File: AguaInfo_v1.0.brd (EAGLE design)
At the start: 100 x 80 mm, 10 parts

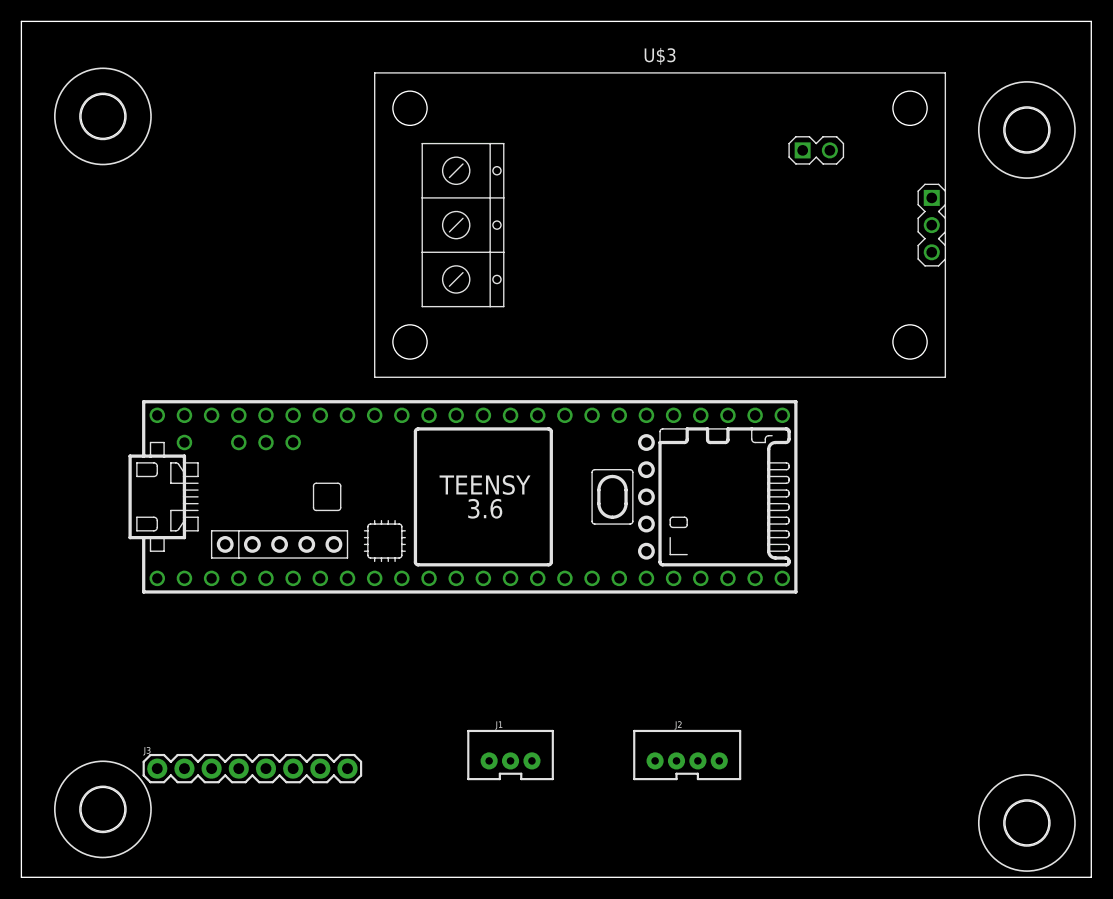
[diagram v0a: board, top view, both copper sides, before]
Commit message: changed Version on PC
All the chages at once.
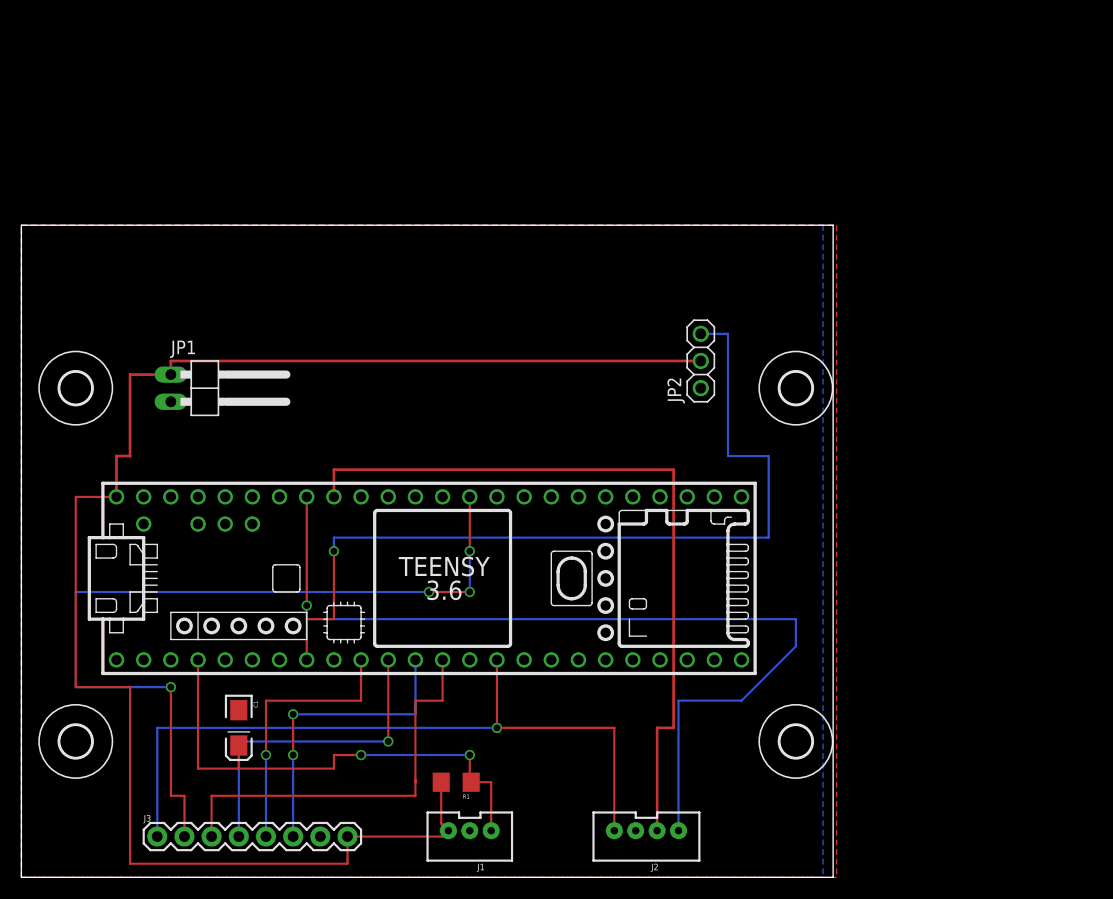
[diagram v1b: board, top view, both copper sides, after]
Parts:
- removed FRAME1: FRAME-LETTER, SparkFun-Retired:CREATIVE_COMMONS
- removed U$3: RELAY-1-SRD, diy-modules:RELAY-1-SRD
- added C1: 0.1uF, SparkFun-Passives:EIA3216-KIT
- added JP1: 5Vin, pinhead:1X02/90
- added JP2: 5v Relay, adafruit:1X03
- added R1: 10K, SparkFun-Resistors:1206
- H1, H2, H3, H4: value MOUNT-HOLE4.1 -> MOUNT-HOLE3.0; device holes:4,1 -> holes:3,0
- J1: value (none) -> WFS
- J2: value (none) -> TOF
- J3: value (none) -> 2.8TFT
- moved H4 105.7 mm to (5.08, 12.7)
- moved H3 97.7 mm to (5.08, 45.7)
- moved H1 87.2 mm to (72.4, 12.7)
- moved H2 75.8 mm to (72.4, 45.7)
- moved J1 8.52 mm to (41.9, 3.81), turned to 180 degrees
- moved U$1 8.52 mm to (36.8, 27.9)
- moved J2 8.52 mm to (58.4, 3.81), turned to 180 degrees
- moved J3 6.35 mm to (12.7, 3.81)
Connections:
- removed net VCC.1: U$3.J1.3
- removed net VCC.2: U$3.J2.2
- new net 3V3: J2.4, J3.1, U$1.3V3
- new net 5V: J1.3, J3.8, JP1.1, JP2.2, R1.2, U$1.VIN
- new net A0: J3.4, U$1.9/CS
- new net CS: J3.6, U$1.10/CS
- new net D6: JP2.3, U$1.6
- new net INT2: C1.A, J1.1, R1.1, U$1.2
- new net MOSI: J3.3, U$1.11/MOSI
- new net RESET: J3.5, U$1.8
- new net SCK: J3.2, U$1.13/SCK
- new net SCL: J2.1, U$1.19/A5/SCL
- new net SDA: J2.2, U$1.18/A4/SDA
- net GND: now also C1.C, J1.2, J2.3, J3.7, JP1.2, JP2.1, U$1.GND; no longer U$3.J1.1
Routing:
- net 5V: track 0.00 -> 147.8 mm
- net SCL: track 0.00 -> 84.9 mm, vias 0 -> 1
- net D6: track 0.00 -> 80.0 mm, vias 0 -> 1
- net SCK: track 0.00 -> 78.7 mm, vias 0 -> 4
- net SDA: track 0.00 -> 69.6 mm
- net 3V3: track 0.00 -> 68.8 mm, vias 0 -> 1
- net INT2: track 0.00 -> 48.1 mm, vias 0 -> 2
- net MOSI: track 0.00 -> 38.3 mm
- net A0: track 0.00 -> 30.5 mm, vias 0 -> 1
- net CS: track 0.00 -> 27.9 mm, vias 0 -> 2
- net RESET: track 0.00 -> 25.4 mm, vias 0 -> 1
- added copper zone on layer 1, net GND
- added copper zone on layer 16, net GND
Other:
- board size 100 x 80 mm -> 75.9 x 61 mm
- board text added: "Aguaingo by Flatbox"
- board text added: "v1.0"
